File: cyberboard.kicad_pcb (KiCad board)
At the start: 4 copper layers, 55 x 55 mm, 55 parts, among them J1 Conn_01x02, J2 USB_C_Receptacle_USB2.0, J3 5024940670, J4 Conn_01x07, J5 Conn_01x07, J6 Conn_01x07, Q1 AO3400A, Q2 AO3400A, Q3 AO3400A, Q5 AO3400A, U2 TJA1051T, U3 D3V3XA4B10LP, U4 TLV75801PDRV, U5 ICM-20948, U6 ESP32-S3-WROOM-1, U7 TLV70018_SOT23-5

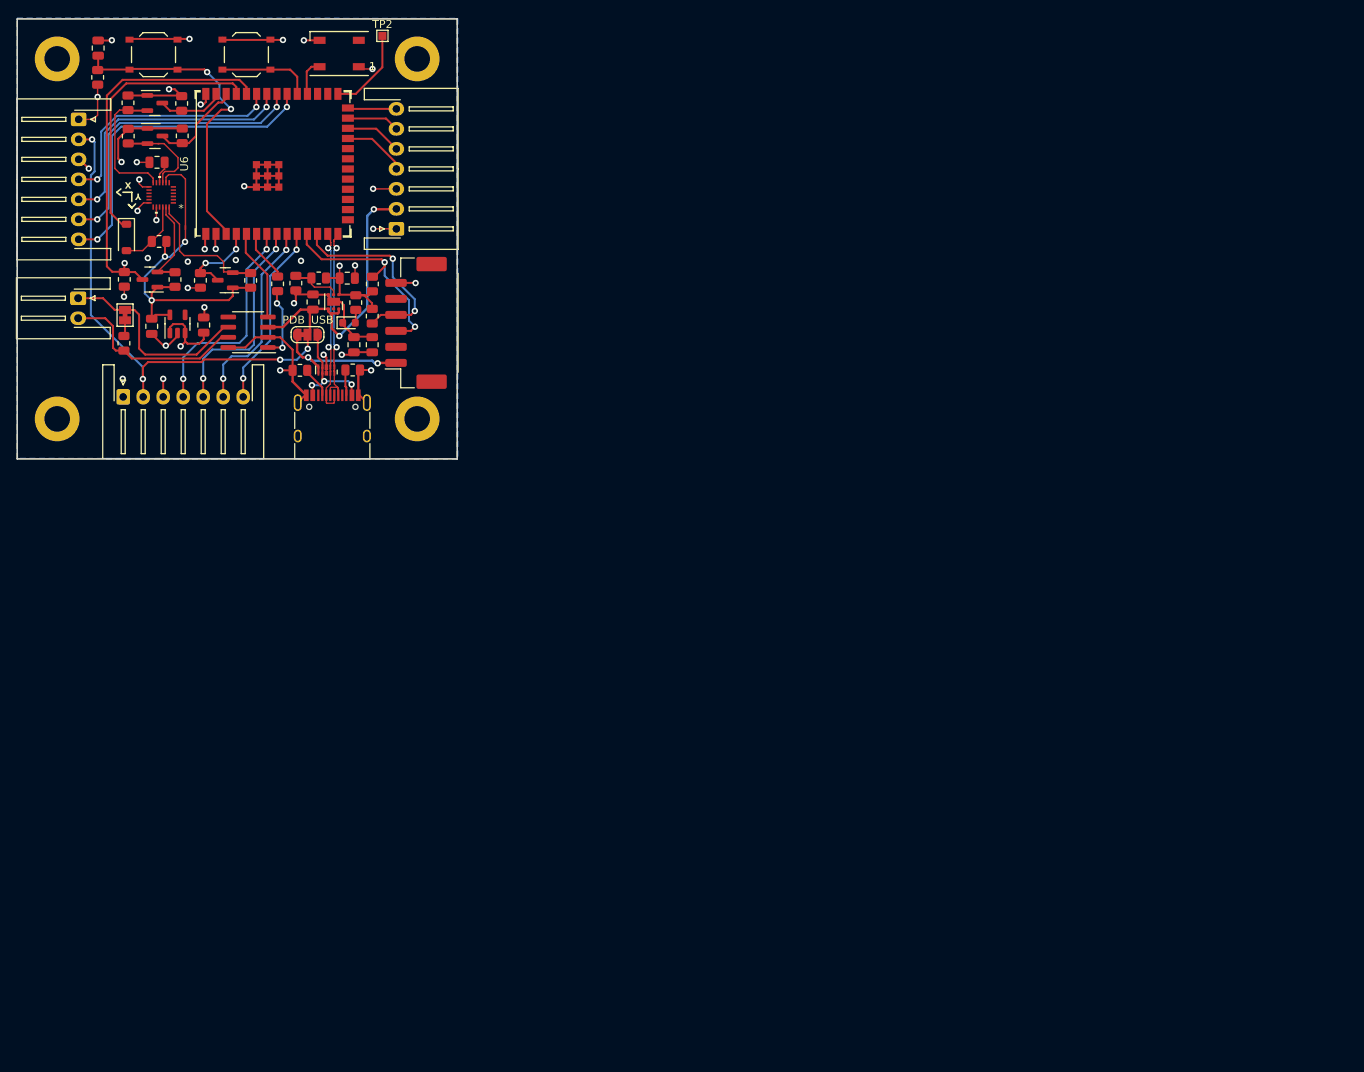
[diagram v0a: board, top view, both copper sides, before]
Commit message: deployment release
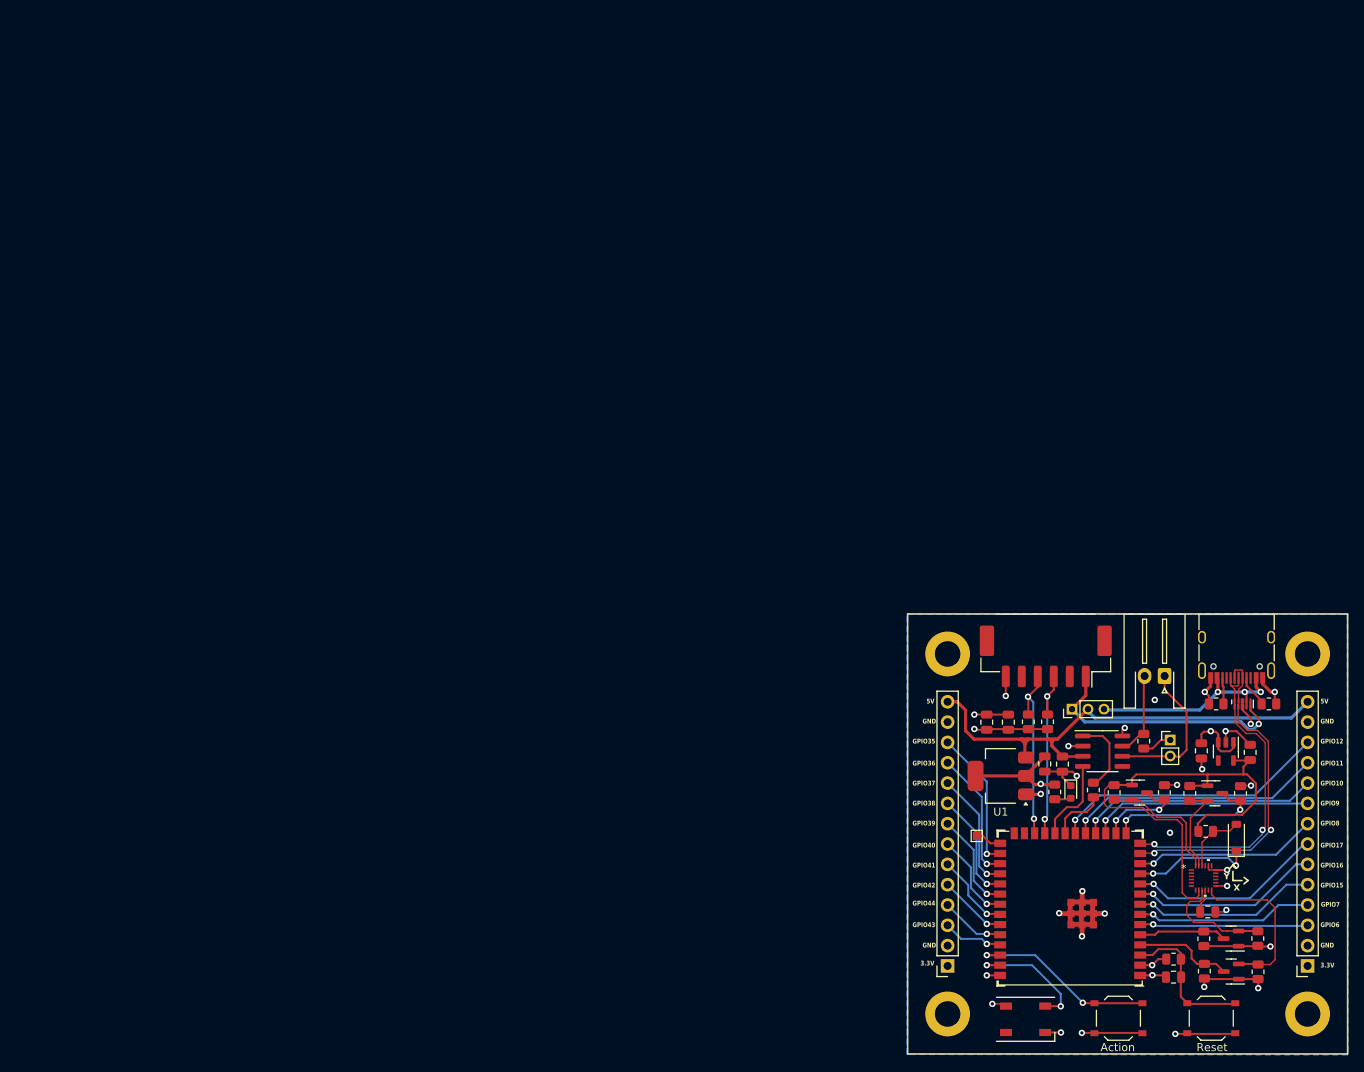
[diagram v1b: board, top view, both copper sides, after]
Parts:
- removed J5, J6: Conn_01x07, Connector_JST:JST_XH_S7B-XH-A-1_1x07_P2.50mm_Horizontal
- removed JP2: SolderJumper_3_Bridged12, Jumper:SolderJumper-3_P1.3mm_Bridged12_RoundedPad1.0x1.5mm_NumberLabels
- removed R6: 1M, Resistor_SMD:R_0805_2012Metric
- removed R7: 200k, Resistor_SMD:R_0805_2012Metric
- removed U4: TLV75801PDRV, Package_SON:WSON-6-1EP_2x2mm_P0.65mm_EP1x1.6mm
- added J8: Conn_01x14, Connector_PinSocket_2.54mm:PinSocket_1x14_P2.54mm_Vertical, F.Cu at (161.3, 118.4)
- added JP3: Jumper_2_Bridged, Connector_PinHeader_2.00mm:PinHeader_1x02_P2.00mm_Vertical, F.Cu at (144.1, 90.1)
- added U1: AMS1117-3.3, Package_TO_SOT_SMD:SOT-223-3_TabPin2, F.Cu at (122.9, 94.6)
- J4: value Conn_01x07 -> Conn_01x14; footprint Connector_JST:JST_XH_S7B-XH-A-1_1x07_P2.50mm_Horizontal -> Connector_PinSocket_2.54mm:PinSocket_1x14_P2.54mm_Vertical
- JP1: value SolderJumper_2_Bridged -> Jumper_3_Bridged12; footprint Jumper:SolderJumper-2_P1.3mm_Bridged_Pad1.0x1.5mm -> Connector_PinHeader_2.00mm:PinHeader_1x03_P2.00mm_Vertical
- moved H2 196.7 mm to (161.3, 124.4), turned to 180 degrees
- moved RESET1 178.9 mm to (149.3, 124.9), turned to 180 degrees
- moved R12 178.2 mm to (155.1, 119.1), turned to 90 degrees
- moved C1 177.6 mm to (144.5, 119.8), turned to 180 degrees
- moved R1 173.9 mm to (144.5, 117.5), turned to 0 degrees
- moved R14 173.2 mm to (155.1, 115.0), turned to 90 degrees
- moved Q1 172.9 mm to (151.8, 119.1), turned to 180 degrees
- moved Q2 167.8 mm to (151.7, 115.0), turned to 180 degrees
- moved R19 167.6 mm to (148.4, 119.0), turned to 90 degrees
- moved ACTION1 162.5 mm to (137.7, 124.9), turned to 180 degrees
- moved R13 162.4 mm to (148.3, 115.0), turned to 90 degrees
- moved C5 161.3 mm to (148.8, 111.6), turned to 0 degrees
- moved H3 159.0 mm to (161.3, 79.4), turned to 180 degrees
- moved D3 157.7 mm to (152.4, 102.3), turned to 90 degrees
- moved U5 155.8 mm to (148.3, 107.4), turned to 0 degrees
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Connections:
- J4 pad 2: +5V -> GND
- J4 pad 3: GND -> /GPIO2_1
- J4 pad 4: /GPIO0_1 -> /GPIO2_2
- J4 pad 5: /GPIO0_2 -> /GPIO2_3
- J4 pad 6: /GPIO0_3 -> /GPIO2_4
- J4 pad 7: /GPIO0_4 -> /GPIO2_5
- JP1 pad 1: Net-(JP1-A) -> /Power/5V_PDB
- JP1 pad 2: Net-(J1-Pin_1) -> +5V
- R2 pad 2: Net-(JP1-A) -> Net-(JP3-A)
- U6 pad 10: /GPIO1_4 -> /GPIO1_5
- U6 pad 11: /I2C_SCL -> /IMU_CS
- U6 pad 12: /I2C_SDA -> /GPIO1_6
- U6 pad 15: unconnected-(U6-GPIO3/TOUCH3/ADC1_CH2-Pad15) -> /IMU_SCL
- U6 pad 16: unconnected-(U6-GPIO46-Pad16) -> /IMU_SDA
- U6 pad 17: unconnected-(U6-GPIO9/TOUCH9/ADC1_CH8/FSPIHD/SUBSPIHD-Pad17) -> /GPIO1_7
- U6 pad 18: unconnected-(U6-GPIO10/TOUCH10/ADC1_CH9/FSPICS0/FSPIIO4/SUBSPICS0-Pad18) -> /GPIO1_8
- U6 pad 19: unconnected-(U6-GPIO11/TOUCH11/ADC2_CH0/FSPID/FSPIIO5/SUBSPID-Pad19) -> /GPIO1_9
- U6 pad 20: unconnected-(U6-GPIO12/TOUCH12/ADC2_CH1/FSPICLK/FSPIIO6/SUBSPICLK-Pad20) -> /GPIO1_10
- U6 pad 21: unconnected-(U6-GPIO13/TOUCH13/ADC2_CH2/FSPIQ/FSPIIO7/SUBSPIQ-Pad21) -> /CAN_RX
- U6 pad 22: unconnected-(U6-GPIO14/TOUCH14/ADC2_CH3/FSPIWP/FSPIDQS/SUBSPIWP-Pad22) -> /CAN_TX
- U6 pad 23: /GPIO0_1 -> /I2C_SCL
- U6 pad 24: /GPIO0_2 -> /I2C_SDA
- U6 pad 25: /GPIO0_3 -> unconnected-(U6-GPIO48/SPICLK_N/SUBSPICLK_N_DIFF-Pad25)
- U6 pad 26: /GPIO0_4 -> unconnected-(U6-GPIO45-Pad26)
- U6 pad 28: unconnected-(U6-SPIIO6/GPIO35/FSPID/SUBSPID-Pad28) -> /GPIO2_10
- U6 pad 29: unconnected-(U6-SPIIO7/GPIO36/FSPICLK/SUBSPICLK-Pad29) -> /GPIO2_9
- U6 pad 30: /GPIO_LED -> /GPIO2_8
- U6 pad 31: /GPIO_ACTION -> /GPIO2_7
- U6 pad 32: /GPIO2_4 -> /GPIO2_6
- U6 pad 33: /GPIO2_3 -> /GPIO2_5
- U6 pad 34: /GPIO2_2 -> /GPIO2_4
- U6 pad 35: /GPIO2_1 -> /GPIO2_3
- U6 pad 36: /IMU_SCL -> /GPIO2_2
- U6 pad 37: /IMU_CS -> /GPIO2_1
- U6 pad 38: /IMU_SDO -> /GPIO_ACTION
- U6 pad 39: /IMU_INT -> /GPIO_LED
- U6 pad 4: /IMU_SDA -> /IMU_INT
- U6 pad 5: /CAN_TX -> /IMU_SDO
- U6 pad 6: /CAN_RX -> /GPIO1_1
- U6 pad 7: /GPIO1_1 -> /GPIO1_2
- U6 pad 8: /GPIO1_2 -> /GPIO1_3
- U6 pad 9: /GPIO1_3 -> /GPIO1_4
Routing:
- net +5V: track 99.6 -> 63.0 mm, vias 6 -> 0
- net /GPIO1_10: track 0.00 -> 34.7 mm, vias 0 -> 1
- net /GPIO1_9: track 0.00 -> 32.4 mm, vias 0 -> 1
- net /GPIO2_4: track 41.0 -> 9.93 mm, vias 2 -> 1
- net /GPIO1_8: track 0.00 -> 29.8 mm, vias 0 -> 1
- net /GPIO2_3: track 37.6 -> 8.65 mm, vias 2 -> 1
- net /GPIO1_7: track 0.00 -> 27.8 mm, vias 0 -> 1
- net /IMU_SCL: track 47.7 -> 20.3 mm, vias 1 -> 2
- net /GPIO2_2: track 34.3 -> 8.11 mm, vias 2 -> 1
- net /GPIO1_5: track 0.00 -> 24.5 mm, vias 0 -> 1
- net /GPIO2_1: track 31.3 -> 7.59 mm, vias 2 -> 1
- net /GPIO1_6: track 0.00 -> 23.0 mm, vias 0 -> 1
- net /EN: track 40.1 -> 18.4 mm, vias 2 -> 0
- net /IMU_CS: track 35.0 -> 15.4 mm, vias 0 -> 2
- net GND: track 106.3 -> 87.9 mm, vias 25 -> 24
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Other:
- board text added: "3.3V"
- board text added: "5V"
- board text added: "Action"
- board text added: "GND"
- board text added: "GPIO10"
- board text added: "GPIO11"
- board text added: "GPIO12"
- board text added: "GPIO15"
- board text added: "GPIO16"
- board text added: "GPIO17"
- board text added: "GPIO35"
- board text added: "GPIO36"
- board text added: "GPIO37"
- board text added: "GPIO38"
- board text added: "GPIO39"
- board text added: "GPIO40"
- board text added: "GPIO41"
- board text added: "GPIO42"
- board text added: "GPIO43"
- board text added: "GPIO44"
- board text added: "GPIO6"
- board text added: "GPIO7"
- board text added: "GPIO8"
- board text added: "GPIO9"
- board text added: "Reset"
